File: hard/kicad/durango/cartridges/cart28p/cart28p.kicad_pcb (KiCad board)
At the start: 2 copper layers, 27.9 x 48.3 mm, 7 parts, among them J1 Edge Connector, U1 27C64/128/256/512

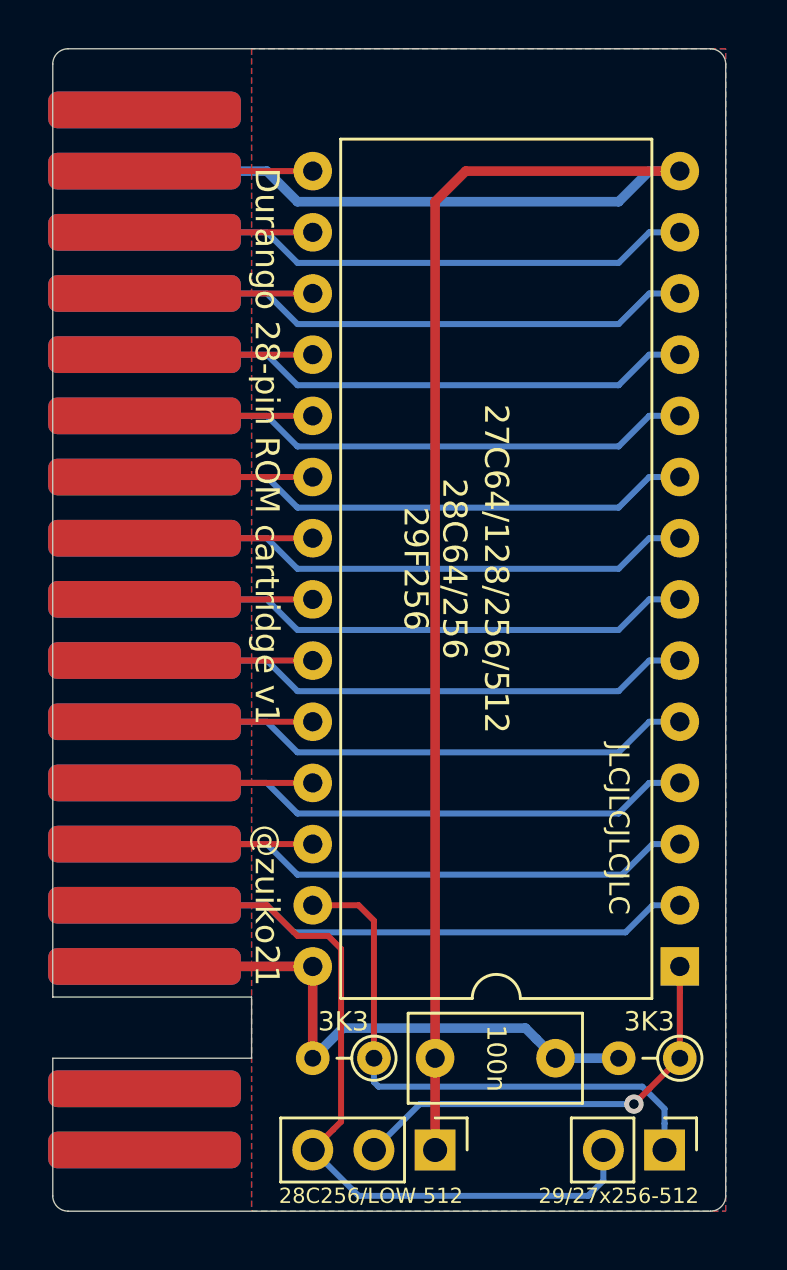
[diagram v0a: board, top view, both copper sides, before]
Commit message: add wrong gerbers for 28p cart
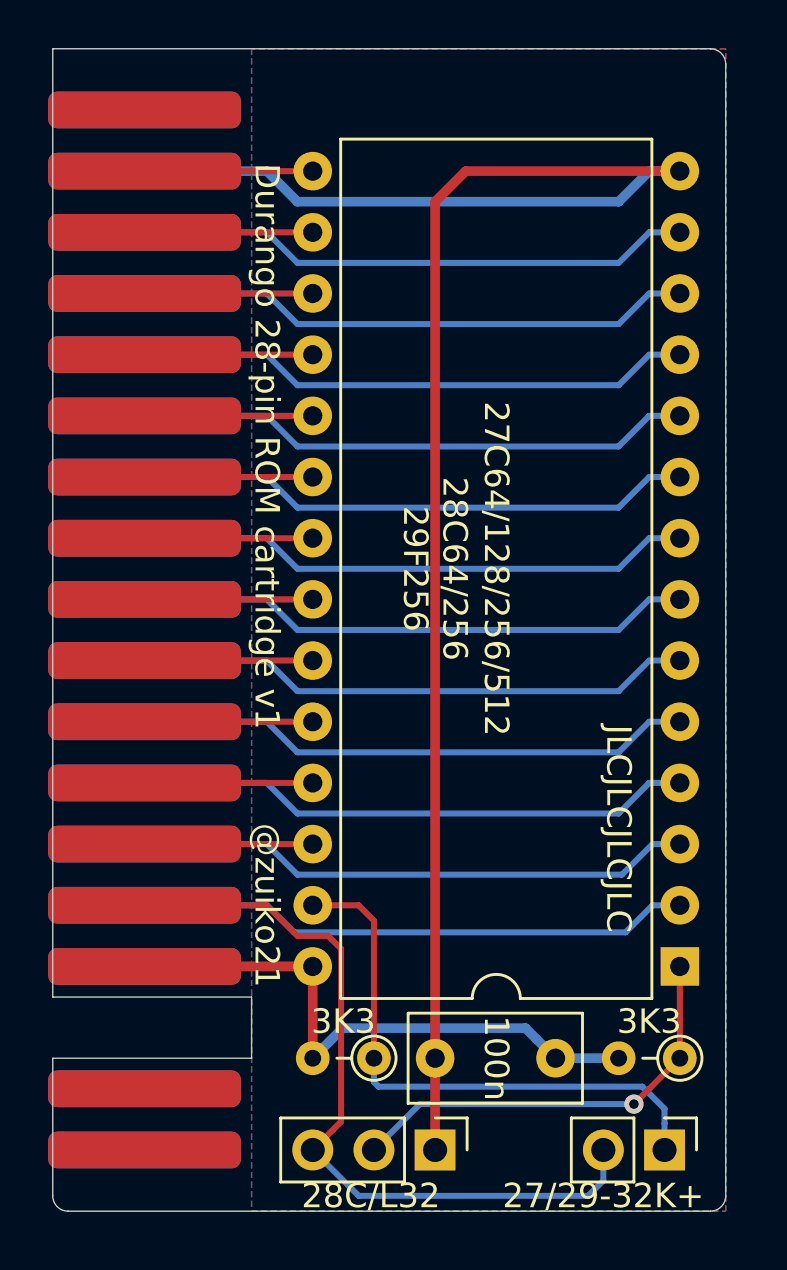
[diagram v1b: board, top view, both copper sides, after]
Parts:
- JP1: value 29/27x256-512 -> 27/29-32K+
- JP2: value 28C256/LOW 512 -> 28C/L32
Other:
- outline, holes or cut-outs redrawn
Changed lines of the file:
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@@
   (general
     (thickness 1.6)
-    (drawings 17)
+    (drawings 16)
     (tracks 115)
     (zones 0)
@@
   (page A4)
   (layers
-    (0 F.Cu signal)
-    (31 B.Cu signal)
-    (32 B.Adhes user)
-    (33 F.Adhes user)
-    (34 B.Paste user)
-    (35 F.Paste user)
-    (36 B.SilkS user)
-    (37 F.SilkS user)
-    (38 B.Mask user)
-    (39 F.Mask user)
-    (40 Dwgs.User user)
-    (41 Cmts.User user)
-    (42 Eco1.User user)
-    (43 Eco2.User user)
+    (0 F.Cu signal hide)
+    (31 B.Cu signal hide)
+    (32 B.Adhes user hide)
+    (33 F.Adhes user hide)
+    (34 B.Paste user hide)
+    (35 F.Paste user hide)
+    (36 B.SilkS user hide)
+    (37 F.SilkS user hide)
+    (38 B.Mask user hide)
+    (39 F.Mask user hide)
+    (40 Dwgs.User user hide)
+    (41 Cmts.User user hide)
+    (42 Eco1.User user hide)
+    (43 Eco2.User user hide)
     (44 Edge.Cuts user)
-    (45 Margin user)
-    (46 B.CrtYd user)
-    (47 F.CrtYd user)
-    (48 B.Fab user)
-    (49 F.Fab user)
+    (45 Margin user hide)
+    (46 B.CrtYd user hide)
+    (47 F.CrtYd user hide)
+    (48 B.Fab user hide)
+    (49 F.Fab user hide)
   )
   (setup
@@
     (pcbplotparams
       (layerselection 0x010fc_ffffffff)
-      (usegerberextensions false)
+      (usegerberextensions true)
       (usegerberattributes false)
       (usegerberadvancedattributes false)
       (creategerberjobfile false)
       (excludeedgelayer true)
-      (linewidth 0.100000)
+      (linewidth 0.150000)
       (plotframeref false)
       (viasonmask false)
@@
       (plotinvisibletext false)
       (padsonsilk false)
-      (subtractmaskfromsilk false)
+      (subtractmaskfromsilk true)
       (outputformat 1)
       (mirror false)
-      (drillshape 1)
+      (drillshape 0)
       (scaleselection 1)
-      (outputdirectory ""))
+      (outputdirectory "gerber/"))
   )
   (net 0 "")
@@
     (at 55.88 27.94 270)
     (fp_text reference J1 (at 2.54 -8.89 unlocked) (layer B.SilkS)
-      (effects (font (size 1 1) (thickness 0.15)) (justify mirror))
+      (effects (font (size 1.016 1.016) (thickness 0.16)) (justify mirror))
     )
     (fp_text value "Edge Connector" (at 24.13 1.27 90) (layer F.Fab)
@@
     (tags "THT DIP DIL PDIP 2.54mm 15.24mm 600mil")
     (fp_text reference U1 (at 7.493 16.51 unlocked) (layer B.SilkS)
-      (effects (font (size 1 1) (thickness 0.15)) (justify mirror))
+      (effects (font (size 1.016 1.016) (thickness 0.16)) (justify mirror))
     )
     (fp_text value 27C64/128/256/512 (at 7.62 16.51 270 unlocked) (layer F.SilkS)
-      (effects (font (size 1 1) (thickness 0.15)))
+      (effects (font (size 1.016 1.016) (thickness 0.16)))
     )
     (fp_arc (start 7.62 -1.33) (end 6.62 -1.33) (angle -180) (layer F.SilkS) (width 0.12))
@@
     (tags "C Rect series Radial pin pitch 5.00mm  length 7mm width 3.5mm Capacitor")
     (fp_text reference C1 (at 2.5 0) (layer B.SilkS)
-      (effects (font (size 1 1) (thickness 0.15)) (justify mirror))
+      (effects (font (size 1 1) (thickness 0.16)) (justify mirror))
     )
     (fp_text value 100n (at 2.54 0 270 unlocked) (layer F.SilkS)
-      (effects (font (size 0.8 0.8) (thickness 0.12)))
+      (effects (font (size 1.016 1.016) (thickness 0.16)))
     )
     (fp_text user %R (at 2.5 0) (layer F.Fab)
-      (effects (font (size 1 1) (thickness 0.15)))
+      (effects (font (size 1 1) (thickness 0.16)))
     )
     (fp_line (start 6.25 -2) (end -1.25 -2) (layer F.CrtYd) (width 0.05))
@@
     (tags "Resistor Axial_DIN0204 series Axial Vertical pin pitch 2.54mm 0.167W length 3.6mm diameter 1.6mm")
     (fp_text reference R2 (at 1.27 1.524 unlocked) (layer B.SilkS)
-      (effects (font (size 1 1) (thickness 0.15)) (justify mirror))
+      (effects (font (size 1.016 1.016) (thickness 0.16)) (justify mirror))
     )
     (fp_text value 3K3 (at 1.27 1.524 unlocked) (layer F.SilkS)
-      (effects (font (size 0.8 0.8) (thickness 0.12)))
+      (effects (font (size 1.016 1.016) (thickness 0.16)))
     )
     (fp_text user %R (at 1.27 -1.92) (layer F.Fab)
@@
     (tags "Resistor Axial_DIN0204 series Axial Vertical pin pitch 2.54mm 0.167W length 3.6mm diameter 1.6mm")
     (fp_text reference R1 (at 1.27 1.524) (layer B.SilkS)
-      (effects (font (size 1 1) (thickness 0.15)) (justify mirror))
+      (effects (font (size 1.016 1.016) (thickness 0.16)) (justify mirror))
     )
     (fp_text value 3K3 (at 1.27 1.524 unlocked) (layer F.SilkS)
-      (effects (font (size 0.8 0.8) (thickness 0.12)))
+      (effects (font (size 1.016 1.016) (thickness 0.16)))
     )
     (fp_text user %R (at 1.27 -1.92) (layer F.Fab)
@@
     (tags "Through hole pin header THT 1x03 2.54mm single row")
     (fp_text reference JP2 (at -1.778 2.413 unlocked) (layer B.SilkS)
-      (effects (font (size 1 1) (thickness 0.15)) (justify mirror))
-    )
-    (fp_text value "28C256/LOW 512" (at 1.905 2.667 unlocked) (layer F.SilkS)
-      (effects (font (size 0.635 0.635) (thickness 0.1)))
+      (effects (font (size 1.016 1.016) (thickness 0.16)) (justify mirror))
+    )
+    (fp_text value 28C/L32 (at 1.905 2.667 unlocked) (layer F.SilkS)
+      (effects (font (size 1.016 1.016) (thickness 0.153)))
     )
     (fp_text user %R (at 0 2.54) (layer F.Fab)
@@
     (tags "Through hole pin header THT 1x02 2.54mm single row")
     (fp_text reference JP1 (at -1.778 1.27 unlocked) (layer B.SilkS)
-      (effects (font (size 1 1) (thickness 0.15)) (justify mirror))
-    )
-    (fp_text value 29/27x256-512 (at 1.905 1.905 unlocked) (layer F.SilkS)
-      (effects (font (size 0.635 0.635) (thickness 0.1)))
+      (effects (font (size 1.016 1.016) (thickness 0.16)) (justify mirror))
+    )
+    (fp_text value 27/29-32K+ (at 1.905 2.54 unlocked) (layer F.SilkS)
+      (effects (font (size 1.016 1.016) (thickness 0.153)))
     )
     (fp_text user %R (at 0 1.27) (layer F.Fab)
@@
   )
   (gr_text "28C64/256\n29F256" (at 71.755 49.53 270) (layer F.SilkS)
-    (effects (font (size 1 1) (thickness 0.15)))
+    (effects (font (size 1.016 1.016) (thickness 0.16)))
   )
   (gr_text JLCJLCJLCJLC (at 79.375 60.325 270) (layer F.SilkS)
-    (effects (font (size 0.84 0.84) (thickness 0.1575)))
+    (effects (font (size 1.016 1.016) (thickness 0.1575)))
   )
   (gr_arc (start 83.185 75.565) (end 83.185 76.2) (angle -90) (layer Edge.Cuts) (width 0.05))
   (gr_arc (start 56.515 75.565) (end 55.88 75.565) (angle -90) (layer Edge.Cuts) (width 0.05))
-  (gr_arc (start 56.515 28.575) (end 56.515 27.94) (angle -90) (layer Edge.Cuts) (width 0.05))
   (gr_arc (start 56.515 28.575) (end 56.515 27.94) (angle 0) (layer Edge.Cuts) (width 0.05))
   (gr_arc (start 83.185 28.575) (end 83.82 28.575) (angle -90) (layer Edge.Cuts) (width 0.05))
   (gr_text @zuiko21 (at 64.77 63.5 270) (layer F.SilkS)
-    (effects (font (size 1 1) (thickness 0.18)))
+    (effects (font (size 1.016 1.016) (thickness 0.18)))
   )
   (gr_text "Durango 28-pin ROM cartridge v1" (at 64.77 44.45 270) (layer F.SilkS)
-    (effects (font (size 1 1) (thickness 0.15)))
+    (effects (font (size 1.016 1.016) (thickness 0.16)))
   )
   (gr_line (start 55.88 69.85) (end 55.88 75.565) (layer Edge.Cuts) (width 0.05))
@@
   (gr_line (start 64.135 67.31) (end 64.135 69.85) (layer Edge.Cuts) (width 0.05))
   (gr_line (start 55.88 67.31) (end 64.135 67.31) (layer Edge.Cuts) (width 0.05))
-  (gr_line (start 55.88 28.575) (end 55.88 67.31) (layer Edge.Cuts) (width 0.05))
-  (gr_line (start 83.185 27.94) (end 56.515 27.94) (layer Edge.Cuts) (width 0.05))
+  (gr_line (start 55.88 27.94) (end 55.88 67.31) (layer Edge.Cuts) (width 0.05))
+  (gr_line (start 83.185 27.94) (end 55.88 27.94) (layer Edge.Cuts) (width 0.05))
   (gr_line (start 83.82 75.565) (end 83.82 28.575) (layer Edge.Cuts) (width 0.05))
   (gr_line (start 56.515 76.2) (end 83.185 76.2) (layer Edge.Cuts) (width 0.05))
